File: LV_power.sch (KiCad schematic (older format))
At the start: 36 parts, among them T1 7508110151, U4 TPS76201, U5 TPS76201, U6 XCL221B18, U7 VIPER26HD

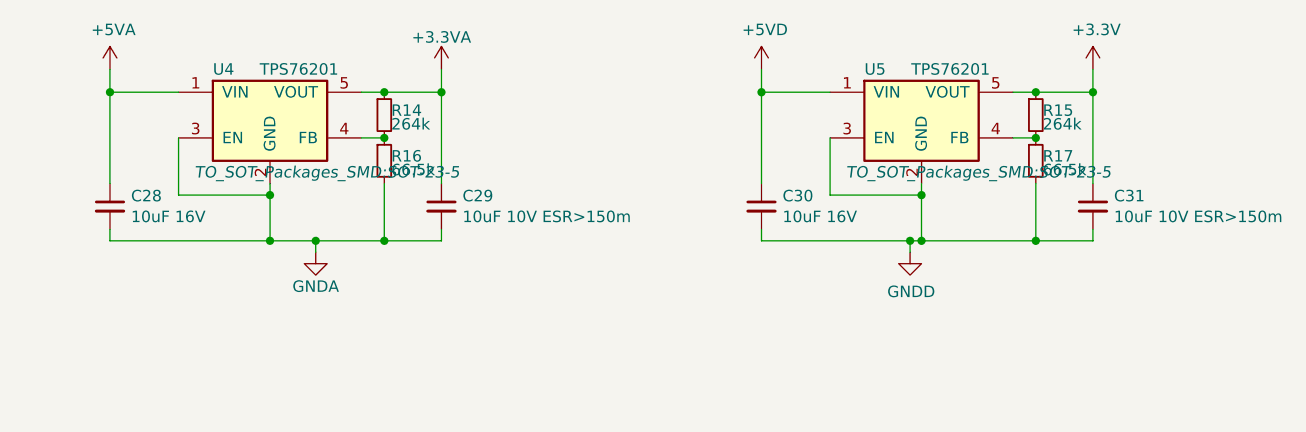
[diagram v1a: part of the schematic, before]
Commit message: As sent to Tempo 2016-10-21
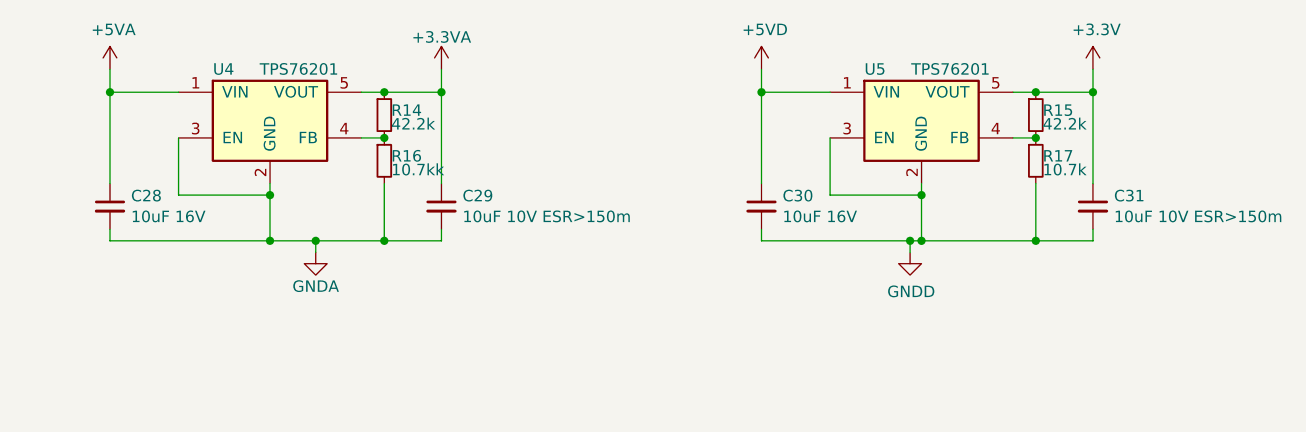
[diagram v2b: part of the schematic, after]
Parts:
- R14, R15: value 264k -> 42.2k
- R16: value 66.5k -> 10.7kk
- R17: value 66.5k -> 10.7k
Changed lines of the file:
@@
 F 0 "U5" H 8350 1200 50  0000 L CNN
 F 1 "TPS76201" H 8900 1200 50  0000 R CNN
-F 2 "TO_SOT_Packages_SMD:SOT-23-5" H 8850 750 50  0000 C CIN
+F 2 "TO_SOT_Packages_SMD:SOT-23-5" H 8850 750 50  0001 C CIN
 F 3 "" H 8600 1000 50  0000 C CNN
 	1    8600 1000
@@
 P 9100 1000
 F 0 "R15" H 9130 1020 50  0000 L CNN
-F 1 "264k" H 9130 960 50  0000 L CNN
+F 1 "42.2k" H 9130 960 50  0000 L CNN
 F 2 "Resistors_SMD:R_0402" H 9100 1000 50  0001 C CNN
 F 3 "" H 9100 1000 50  0000 C CNN
@@
 P 9100 1200
 F 0 "R17" H 9130 1220 50  0000 L CNN
-F 1 "66.5k" H 9130 1160 50  0000 L CNN
+F 1 "10.7k" H 9130 1160 50  0000 L CNN
 F 2 "Resistors_SMD:R_0402" H 9100 1200 50  0001 C CNN
 F 3 "" H 9100 1200 50  0000 C CNN
@@
 F 0 "U4" H 5500 1200 50  0000 L CNN
 F 1 "TPS76201" H 6050 1200 50  0000 R CNN
-F 2 "TO_SOT_Packages_SMD:SOT-23-5" H 6000 750 50  0000 C CIN
+F 2 "TO_SOT_Packages_SMD:SOT-23-5" H 6000 750 50  0001 C CIN
 F 3 "" H 5750 1000 50  0000 C CNN
 	1    5750 1000
@@
 P 6250 1000
 F 0 "R14" H 6280 1020 50  0000 L CNN
-F 1 "264k" H 6280 960 50  0000 L CNN
+F 1 "42.2k" H 6280 960 50  0000 L CNN
 F 2 "Resistors_SMD:R_0402" H 6250 1000 50  0001 C CNN
 F 3 "" H 6250 1000 50  0000 C CNN
@@
 P 6250 1200
 F 0 "R16" H 6280 1220 50  0000 L CNN
-F 1 "66.5k" H 6280 1160 50  0000 L CNN
+F 1 "10.7kk" H 6280 1160 50  0000 L CNN
 F 2 "Resistors_SMD:R_0402" H 6250 1200 50  0001 C CNN
 F 3 "" H 6250 1200 50  0000 C CNN
